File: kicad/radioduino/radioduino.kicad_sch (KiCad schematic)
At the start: 0 parts

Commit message: basic schematic
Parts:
- added A1: Arduino_Nano_v3.x, Module:Arduino_Nano, symbol MCU_Module:Arduino_Nano_v3.x
- added C1, C2, C3: 100n, Capacitor_SMD:C_0805_2012Metric, symbol Device:C
- added C4, C5: 470n, Capacitor_SMD:C_0805_2012Metric, symbol Device:C
- added C6: 10u, Capacitor_SMD:C_0805_2012Metric, symbol Device:C
- added DS1: WC1602A, Display:WC1602A, symbol Display_Character:WC1602A
- added J1: Conn_01x03_Socket, Connector_PinHeader_2.54mm:PinHeader_1x03_P2.54mm_Vertical, symbol Connector:Conn_01x03_Socket
- added J2, J3, J4, J5: Conn_Coaxial_Small, Connector_Coaxial:SMA_Amphenol_132289_EdgeMount, symbol Connector:Conn_Coaxial_Small
- added J6, J7: Conn_01x15, Connector_PinHeader_2.54mm:PinHeader_1x15_P2.54mm_Vertical, symbol Connector_Generic:Conn_01x15
- added JP1, JP2, JP3, JP8: SolderJumper_2_Open, Jumper:SolderJumper-2_P1.3mm_Open_TrianglePad1.0x1.5mm, symbol Jumper:SolderJumper_2_Open
- added JP4, JP6, JP7: SolderJumper_2_Bridged, Jumper:SolderJumper-2_P1.3mm_Bridged_Pad1.0x1.5mm, symbol Jumper:SolderJumper_2_Bridged
- added JP5: SolderJumper_3_Open, Jumper:SolderJumper-3_P1.3mm_Open_Pad1.0x1.5mm, symbol Jumper:SolderJumper_3_Open
- added Q1: SS8050, Package_TO_SOT_SMD:SOT-23, symbol Transistor_BJT:SS8050
- added Q2, Q3: BSS138, Package_TO_SOT_SMD:SOT-23, symbol Transistor_FET:BSS138
- added R1, R10, R11, R12, R2, R3, R7, R8, R9: 10K, Resistor_SMD:R_0805_2012Metric_Pad1.20x1.40mm_HandSolder, symbol Device:R
- added R4, R5, R6: 4.7K, Resistor_SMD:R_0805_2012Metric_Pad1.20x1.40mm_HandSolder, symbol Device:R
- added RV1: R_Potentiometer, Potentiometer_THT:Potentiometer_Runtron_RM-065_Vertical, symbol Device:R_Potentiometer
- added SW1: RotaryEncoder_Switch_MP, Rotary_Encoder:RotaryEncoder_Alps_EC11E-Switch_Vertical_H20mm, symbol Device:RotaryEncoder_Switch_MP
- added U1: PCF8574AT, Package_SO:SOIC-16W_7.5x10.3mm_P1.27mm, symbol Interface_Expansion:PCF8574AT
- added U2: RT9193-33GB, SOT-23-5_RIT, symbol rt9193:RT9193-33GB
- added Y1: Si5351A-B-GT, Package_SO:MSOP-10_3x3mm_P0.5mm, symbol Oscillator:Si5351A-B-GT
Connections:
- new net: J1.2 (Pin_2), JP5.2 (C)
- new net: A1.30 (VIN), J7.15 (Pin_15), JP5.3 (B)
- new net: C3.1, JP7.1 (A)
- new net: C2.2, C3.2, Y1.2 (XA)
- new net: JP2.2 (B), R2.2, U1.2 (A1)
- new net: JP3.2 (B), R3.2, U1.3 (A2)
- new net: A1.10 (D7), J6.10 (Pin_10), R12.1, SW1.B
- new net: Q1.1 (B), R6.2, U1.7 (P3)
- new net: Q3.3 (D), R10.2, Y1.5 (SDA)
- new net: J3.1 (In), Y1.10 (CLK0)
- new net: Q2.3 (D), R9.2, Y1.4 (SCL)
- new net: J5.1 (In), Y1.6 (CLK2)
- new net: J4.1 (In), Y1.9 (CLK1)
- new net: A1.24 (A5), J7.9 (Pin_9), Q2.2 (S), R5.2, R7.2, U1.14 (SCL)
- new net: DS1.3 (VO), RV1.2
- new net: JP1.2 (B), R1.2, U1.1 (A0)
- new net: A1.16 (D13), J7.1 (Pin_1)
- new net: A1.25 (A6), J7.10 (Pin_10)
- new net: A1.26 (A7), J7.11 (Pin_11)
- new net: A1.27 (+5V), J7.12 (Pin_12), JP4.1 (A)
- new net: A1.28 (~{RESET}), J7.13 (Pin_13)
- new net: A1.18 (AREF), J7.3 (Pin_3)
- new net: A1.19 (A0), J7.4 (Pin_4)
- new net: A1.20 (A1), J7.5 (Pin_5)
- new net: A1.21 (A2), J7.6 (Pin_6)
- new net: A1.22 (A3), J7.7 (Pin_7)
- new net: A1.23 (A4), J7.8 (Pin_8), Q3.2 (S), R4.2, R8.1, U1.15 (SDA)
- new net: A1.9 (D6), J6.9 (Pin_9), R11.1, SW1.A
- new net: A1.1 (D1/TX), J6.1 (Pin_1)
- new net: A1.11 (D8), J6.11 (Pin_11), SW1.S1
- new net: A1.12 (D9), J6.12 (Pin_12)
- new net: A1.13 (D10), J6.13 (Pin_13)
- new net: A1.14 (D11), J6.14 (Pin_14)
- new net: A1.15 (D12), J6.15 (Pin_15)
- new net: A1.2 (D0/RX), J6.2 (Pin_2)
- new net: A1.3 (~{RESET}), J6.3 (Pin_3)
- new net: A1.5 (D2), J6.5 (Pin_5)
- new net: A1.6 (D3), J6.6 (Pin_6)
- new net: A1.7 (D4), J6.7 (Pin_7)
- new net: A1.8 (D5), J6.8 (Pin_8)
- new net: DS1.15 (LED(+)), JP6.2 (B)
- new net: DS1.12 (D5), U1.10 (P5)
- new net: DS1.13 (D6), U1.11 (P6)
- new net: DS1.14 (D7), U1.12 (P7)
- new net: DS1.4 (RS), U1.4 (P0)
- new net: DS1.5 (R/W), U1.5 (P1)
- new net: DS1.6 (E), U1.6 (P2)
- new net: DS1.11 (D4), U1.9 (P4)
- new net: J2.1 (In), JP8.1 (A)
- new net: C2.1, JP8.2 (B)
- new net: DS1.16 (LED(-)), Q1.3 (C)
- new net +3.3V: C4.2, C5.1, Q2.1 (G), Q3.1 (G), R10.1, R9.1, U2.5 (VOUT), Y1.1 (VDD), Y1.7 (VDDO)
- new net +5V: C1.1, C6.1, DS1.2 (VDD), JP4.2 (B), JP5.1 (A), JP6.1 (A), R1.1, R11.2, R12.2, R2.1, R3.1, R4.1, R5.1, R6.1, R7.1, R8.2, RV1.1, U2.1 (VIN), U2.3 (EN)
- new net GND: A1.29 (GND), A1.4 (GND), C1.2, C4.1, C5.2, C6.2, DS1.1 (VSS), J1.1 (Pin_1), J1.3 (Pin_3), J2.2 (Ext), J3.2 (Ext), J4.2 (Ext), J5.2 (Ext), J6.4 (Pin_4), J7.14 (Pin_14), J7.2 (Pin_2), JP1.1 (A), JP2.1 (A), JP3.1 (A), Q1.2 (E), RV1.3, SW1.C, SW1.S2, U2.2 (GND)
- no-connect marks 0 -> 1
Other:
- company: (none) -> YO3DBZ
- title: (none) -> Radioduino

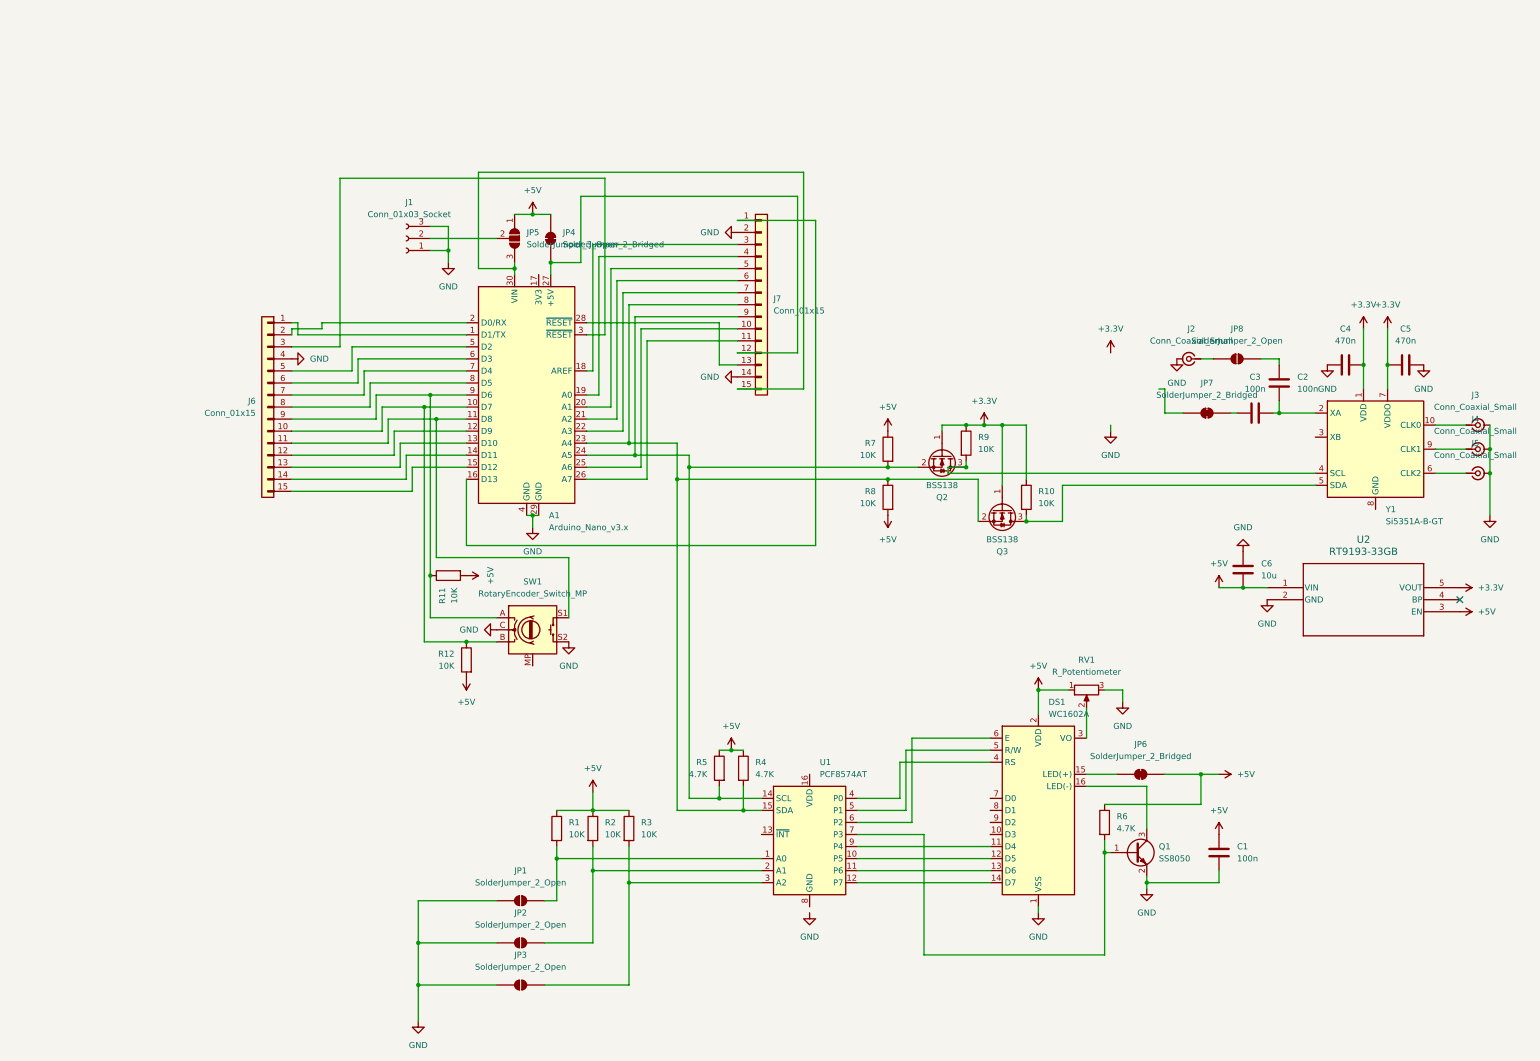
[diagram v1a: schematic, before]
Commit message: made pcb
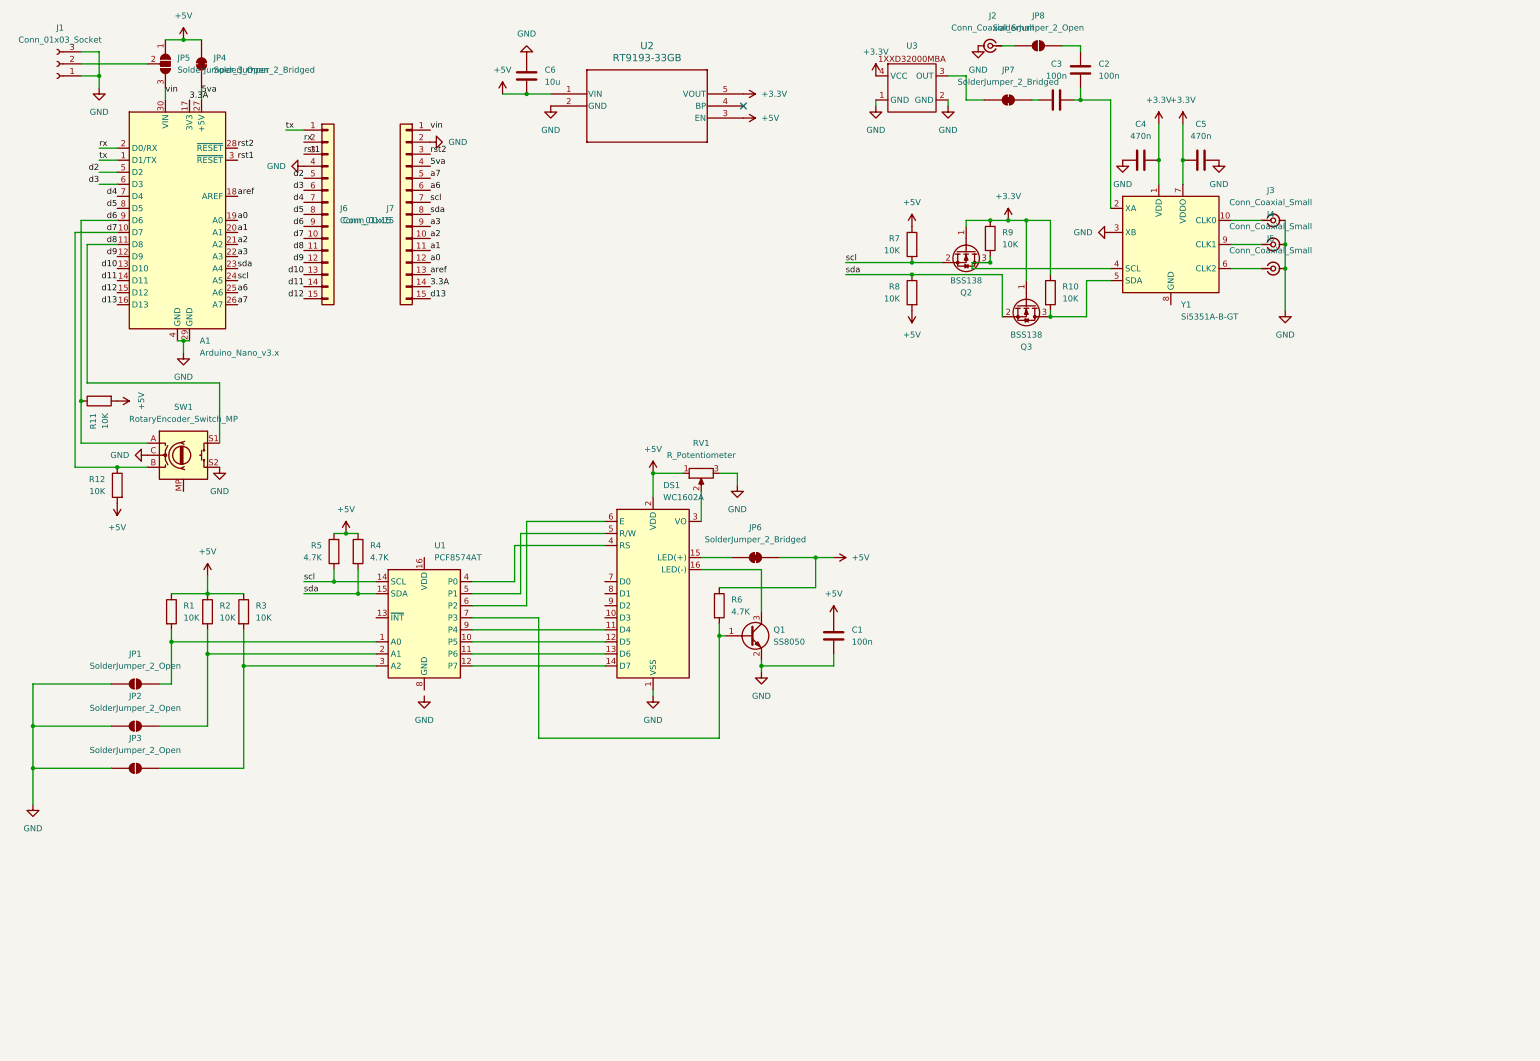
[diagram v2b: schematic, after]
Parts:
- added U3: (no value), Crystal:Crystal_SMD_2016-4Pin_2.0x1.6mm, symbol radioduino:1XXD32000MBA
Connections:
- net +3.3V: now also U3.4 (VCC)
- net GND: now also Y1.3 (XB), U3.1 (GND), U3.2 (GND); no longer J7.14 (Pin_14)
- net vin: now reaches A1.30 (VIN), JP5.3 (B)
- net vin: now also J7.1 (Pin_1); no longer J7.15 (Pin_15)
- net d7: now reaches A1.10 (D7), J6.10 (Pin_10), R12.1, SW1.B
- net at JP7.2 (B): now also U3.3 (OUT)
- net scl: now reaches A1.24 (A5), Q2.2 (S), R5.2, R7.2, U1.14 (SCL)
- net scl: now also J7.7 (Pin_7); no longer J7.9 (Pin_9)
- net d13: now reaches A1.16 (D13)
- net d13: now also J7.15 (Pin_15); no longer J7.1 (Pin_1)
- net a2: now reaches J7.10 (Pin_10)
- net a2: now also A1.21 (A2); no longer A1.25 (A6)
- net a1: now reaches J7.11 (Pin_11)
- net a1: now also A1.20 (A1); no longer A1.26 (A7)
- net 5va: now reaches A1.27 (+5V), JP4.1 (A)
- net 5va: now also J7.4 (Pin_4); no longer J7.12 (Pin_12)
- net aref: now reaches J7.13 (Pin_13)
- net aref: now also A1.18 (AREF); no longer A1.28 (~{RESET})
- net rst2: now reaches J7.3 (Pin_3)
- net rst2: now also A1.28 (~{RESET}); no longer A1.18 (AREF)
- net a0: now reaches A1.19 (A0)
- net a0: now also J7.12 (Pin_12); no longer J7.4 (Pin_4)
- net a7: now reaches J7.5 (Pin_5)
- net a7: now also A1.26 (A7); no longer A1.20 (A1)
- net a6: now reaches J7.6 (Pin_6)
- net a6: now also A1.25 (A6); no longer A1.21 (A2)
- net a3: now reaches A1.22 (A3)
- net a3: now also J7.9 (Pin_9); no longer J7.7 (Pin_7)
- net sda: now reaches A1.23 (A4), J7.8 (Pin_8), Q3.2 (S), R4.2, R8.1, U1.15 (SDA)
- net d6: now reaches A1.9 (D6), J6.9 (Pin_9), R11.1, SW1.A
- net tx: now reaches A1.1 (D1/TX), J6.1 (Pin_1)
- net d8: now reaches A1.11 (D8), J6.11 (Pin_11), SW1.S1
- net d9: now reaches A1.12 (D9), J6.12 (Pin_12)
- net d10: now reaches A1.13 (D10), J6.13 (Pin_13)
- net d11: now reaches A1.14 (D11), J6.14 (Pin_14)
- net d12: now reaches A1.15 (D12), J6.15 (Pin_15)
- net rx: now reaches A1.2 (D0/RX), J6.2 (Pin_2)
- net rst1: now reaches A1.3 (~{RESET}), J6.3 (Pin_3)
- net d2: now reaches A1.5 (D2), J6.5 (Pin_5)
- net d3: now reaches A1.6 (D3), J6.6 (Pin_6)
- net d4: now reaches A1.7 (D4), J6.7 (Pin_7)
- net d5: now reaches A1.8 (D5), J6.8 (Pin_8)
- net 3.3A: now reaches A1.17 (3V3)
- net 3.3A: now also J7.14 (Pin_14)
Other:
- moved on the sheet: A1, C1, C2, C3, C4, C5, C6, DS1, J1, J2, J3, J4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

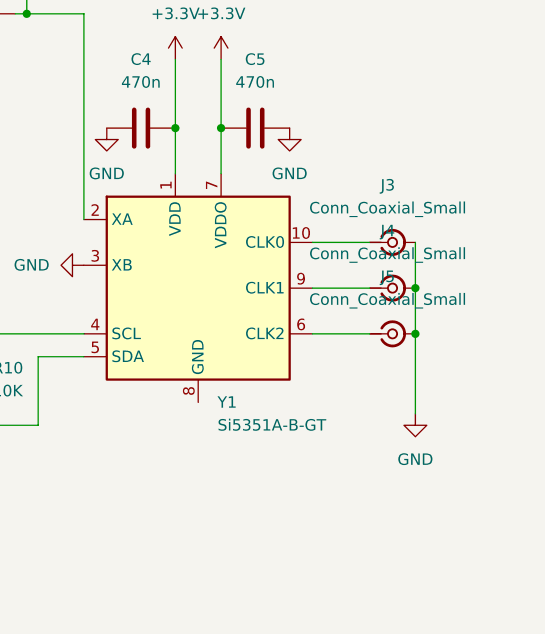
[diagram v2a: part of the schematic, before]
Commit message: pcb
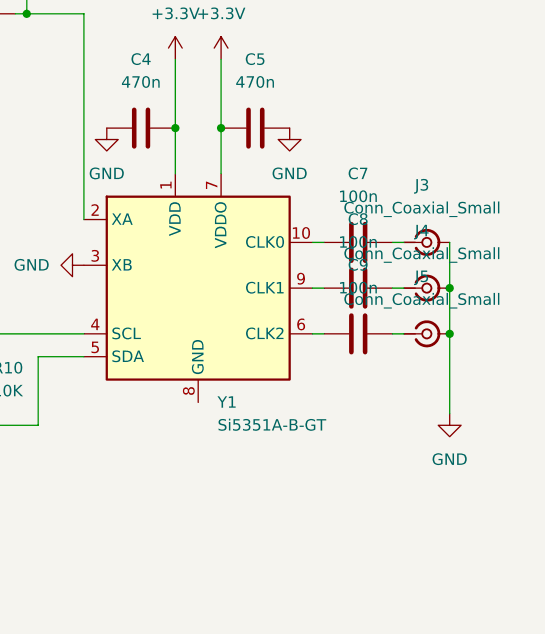
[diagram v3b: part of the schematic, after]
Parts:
- added C7, C8, C9: 100n, Capacitor_SMD:C_0805_2012Metric, symbol Device:C
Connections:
- net at Y1.10 (CLK0): now also C7.1; no longer J3.1 (In)
- net at Y1.6 (CLK2): now also C9.1; no longer J5.1 (In)
- net at Y1.9 (CLK1): now also C8.1; no longer J4.1 (In)
- new net: C9.2, J5.1 (In)
- new net: C8.2, J4.1 (In)
- new net: C7.2, J3.1 (In)
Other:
- moved on the sheet: J3, J4, J5

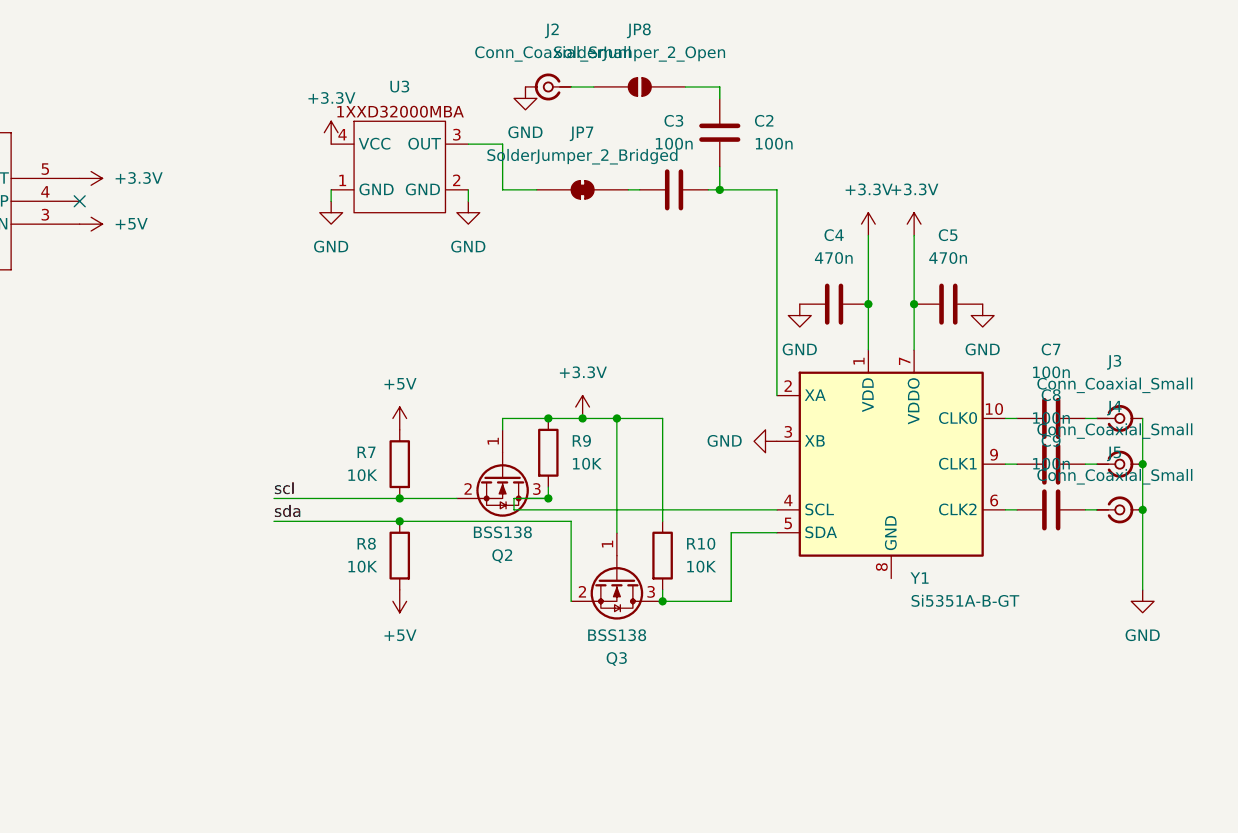
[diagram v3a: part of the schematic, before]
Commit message: before ldo
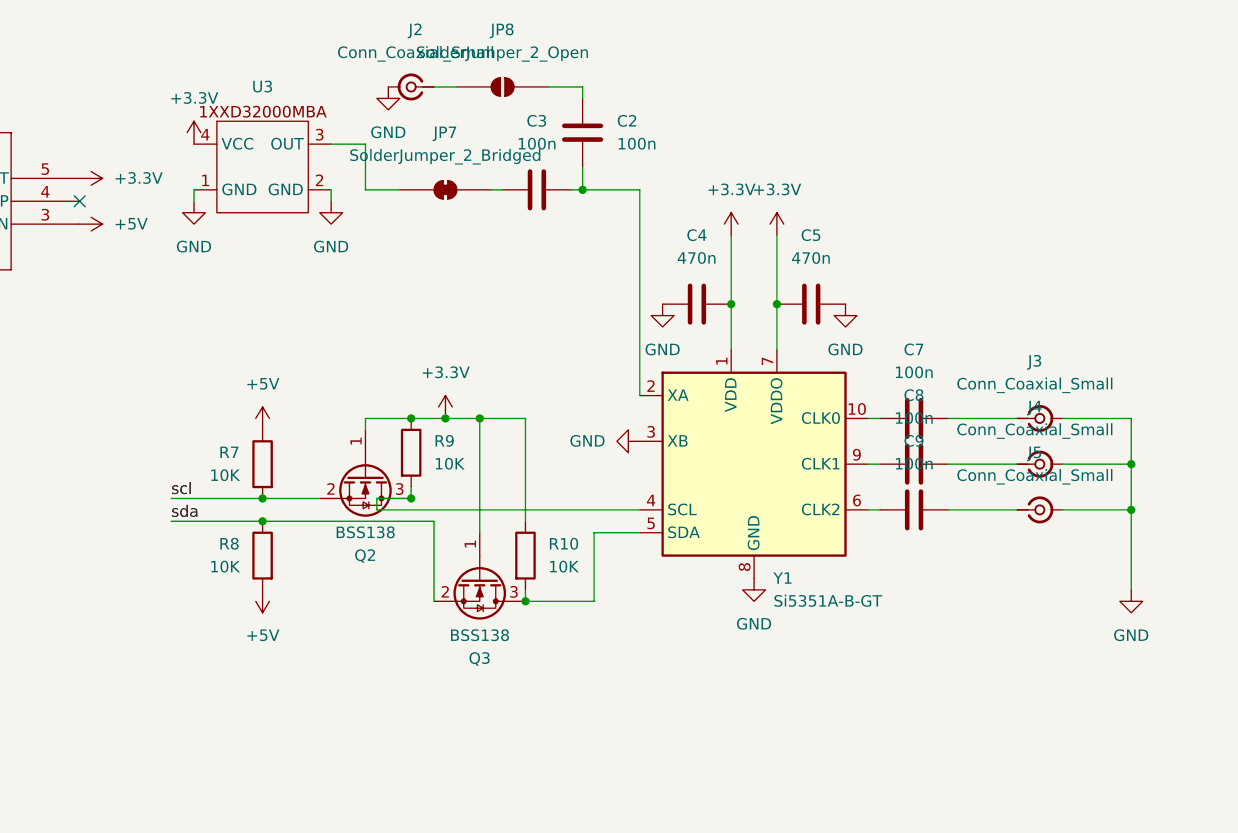
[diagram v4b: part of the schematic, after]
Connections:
- net GND: now also Y1.8 (GND)
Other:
- moved on the sheet: C2, C3, C4, C5, C7, C8, C9, J2, J3, J4, J5, JP7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
